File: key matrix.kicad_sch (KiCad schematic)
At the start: 68 parts, among them J3 JST_SUR_SM04B-SURS-TF, J4 JST_SUR_SM04B-SURS-TF, SW1 SW_Push, SW10 SW_Push, SW11 SW_Push, SW12 SW_Push, SW13 SW_Push, SW14 SW_Push, SW15 SW_Push, SW16 SW_Push, SW17 SW_Push, SW18 SW_Push, SW19 SW_Push, SW2 SW_Push, SW20 SW_Push, SW21 SW_Push, SW22 SW_Push, SW23 SW_Push, SW24 SW_Push, SW25 SW_Push, SW26 SW_Push, SW27 SW_Push, SW28 SW_Push, SW29 SW_Push, SW3 SW_Push, SW30 SW_Push, SW31 SW_Push, SW32 SW_Push, SW33 SW_Push, SW34 SW_Push, SW35 SW_Push, SW36 SW_Push, SW37 SW_Push, SW38 SW_Push, SW39 SW_Push, SW4 SW_Push, SW40 SW_Push, SW41 SW_Push, SW42 SW_Push, SW43 RotaryEncoder_Switch_MP, SW44 RotaryEncoder_Switch_MP, SW49 SW_rocker, SW5 SW_Push, SW50 SW_rocker, SW6 SW_Push, SW7 SW_Push, SW8 SW_Push, SW9 SW_Push, U1 BAT54CTB6_R1_00001, U10 BAT54CTB6_R1_00001, U11 BAT54CTB6_R1_00001, U12 BAT54CTB6_R1_00001, U2 BAT54CTB6_R1_00001, U3 BAT54CTB6_R1_00001, U4 BAT54CTB6_R1_00001, U5 BAT54CTB6_R1_00001, U6 BAT54CTB6_R1_00001, U7 BAT54CTB6_R1_00001, U8 BAT54CTB6_R1_00001, U9 BAT54CTB6_R1_00001

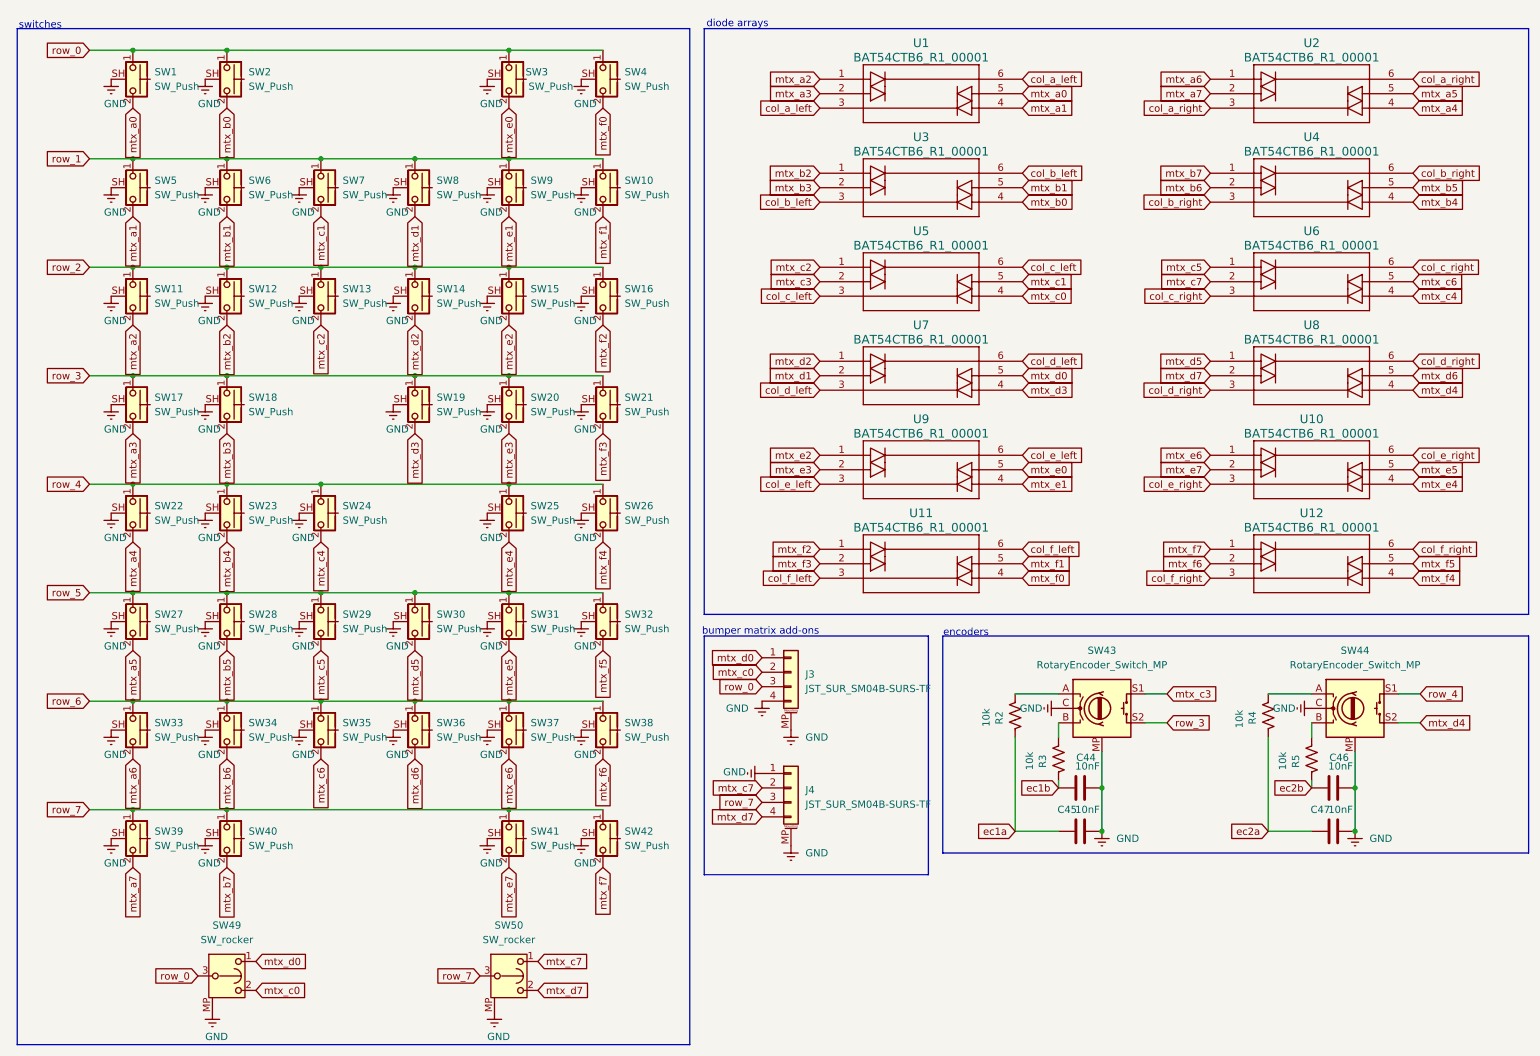
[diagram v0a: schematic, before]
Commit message: v2 final ready to order
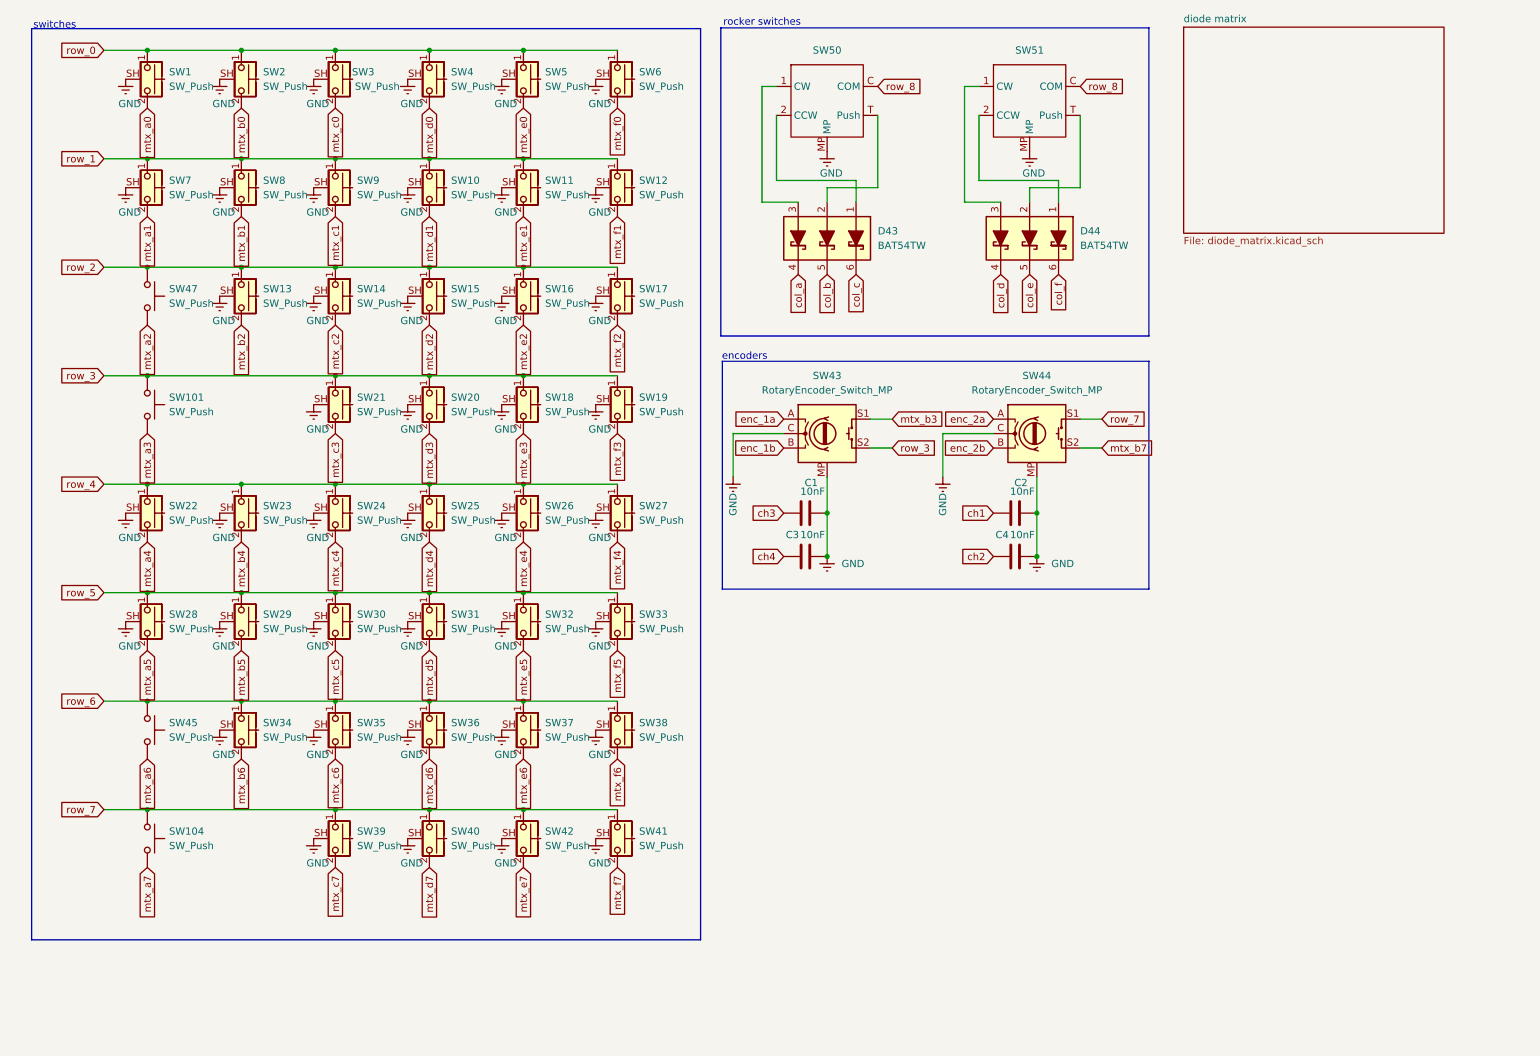
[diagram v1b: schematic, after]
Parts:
- removed C44, C45, C46, C47: 10nF, Capacitor_SMD:C_0603_1608Metric, symbol Device:C
- removed J3, J4: JST_SUR_SM04B-SURS-TF, Connector_JST:JST_SUR_SM04B-SURS-TF_1x04-1MP_P0.80mm_Horizontal, symbol Connector_Generic_MountingPin:Conn_01x04_MountingPin
- removed R2, R3, R4, R5: 10k, Resistor_SMD:R_0603_1608Metric, symbol Device:R_US
- removed SW49, SW50: SW_rocker, coquette_footprints:TMHU27, symbol coquette_symbols:SW_rocker
- removed U1, U10, U11, U12, U2, U3, U4, U5, U6, U7, U8, U9: BAT54CTB6_R1_00001, Package_TO_SOT_SMD:SOT-563, symbol coquette_symbols:BAT54CTB6_R1_00001
- added C1, C2, C3, C4: 10nF, Capacitor_SMD:C_0603_1608Metric, symbol Device:C
- added D43, D44: BAT54TW, PCM_Package_TO_SOT_SMD_AKL:SOT-363_SC-70-6, symbol PCM_Diode_Schottky_AKL:BAT54TW
- added SW101, SW104, SW45, SW47: SW_Push, coquette_footprints:G-Switch GT-TC041B-H036-L1N, symbol Switch:SW_Push
- added SW50, SW51: ~, coquette_footprints:Hanbo WS003, symbol gachlilit:WS-003
- renumbered SW11 to SW10, SW12 to SW11, SW13 to SW12, SW14 to SW13, SW15 to SW14, SW16 to SW15, SW18 to SW16, SW19 to SW18, SW20 to SW19, SW21 to SW20, SW4 to SW21, SW23 to SW22, SW24 to SW23, SW22 to SW24, SW42 to SW27, SW27 to SW28, SW28 to SW29, SW29 to SW30, SW30 to SW31, SW31 to SW32, SW32 to SW33, SW33 to SW34, SW34 to SW35, SW35 to SW36, SW36 to SW37, SW37 to SW38, SW38 to SW39, SW5 to SW4, SW39 to SW40, SW40 to SW41, SW41 to SW42, SW6 to SW5, SW7 to SW6, SW8 to SW7, SW9 to SW8, SW10 to SW9
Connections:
- net GND: now also C1.2, C2.2, C3.2, C4.2, SW50.MP, SW51.MP
- net mtx_a1: now also SW7.2; no longer SW4.2
- net mtx_a2: now also SW47.2; no longer SW10.2
- net mtx_a3: now also SW101.2; no longer SW17.2
- net mtx_a4: now also SW22.2; no longer SW24.2
- net mtx_a6: now also SW45.2; no longer SW34.2
- net mtx_a7: now also SW104.2; no longer SW40.2
- net mtx_b1: now also SW8.2; no longer SW5.2
- net mtx_b2: now also SW13.2; no longer SW11.2
- net mtx_b3: now also SW43.S1; no longer SW16.2
- net mtx_b4: now also SW23.2; no longer SW22.2
- net mtx_b6: now also SW34.2; no longer SW35.2
- net mtx_b7: now also SW44.S2; no longer SW41.2
- net mtx_c0: now also SW3.2
- net mtx_c1: now also SW9.2; no longer SW6.2
- net mtx_c2: now also SW14.2; no longer SW12.2
- net mtx_c3: now also SW21.2; no longer SW43.S1
- net mtx_c4: now also SW24.2; no longer SW23.2
- net mtx_c6: now also SW35.2; no longer SW36.2
- net mtx_c7: now also SW39.2
- net mtx_d0: now also SW4.2
- net mtx_d1: now also SW10.2; no longer SW7.2
- net mtx_d2: now also SW15.2; no longer SW13.2
- net mtx_d3: now also SW20.2; no longer SW18.2
- net mtx_d4: now also SW25.2; no longer SW44.S2
- net mtx_d6: now also SW36.2; no longer SW37.2
- net mtx_d7: now also SW40.2
- net mtx_e0: now also SW5.2; no longer SW3.2
- net mtx_e1: now also SW11.2; no longer SW8.2
- net mtx_e2: now also SW16.2; no longer SW14.2
- net mtx_e3: now also SW18.2; no longer SW19.2
- net mtx_e4: now also SW26.2; no longer SW25.2
- net mtx_e6: now also SW37.2; no longer SW38.2
- net mtx_f0: now also SW6.2; no longer SW21.2
- net mtx_f1: now also SW12.2; no longer SW9.2
- net mtx_f2: now also SW17.2; no longer SW15.2
- net mtx_f3: now also SW19.2; no longer SW20.2
- net mtx_f4: now also SW27.2; no longer SW26.2
- net mtx_f6: now also SW38.2; no longer SW39.2
- net mtx_f7: now also SW41.2; no longer SW27.2
- net row_0: now also SW4.1, SW5.1, SW6.1; no longer SW21.1
- net row_1: now also SW10.1, SW11.1, SW12.1; no longer SW4.1, SW5.1, SW6.1
- net row_2: now also SW16.1, SW17.1, SW47.1; no longer SW10.1, SW11.1, SW12.1
- net row_3: now also SW21.1, SW101.1; no longer SW16.1, SW17.1
- net row_4: now also SW27.1; no longer SW44.S1
- net row_6: now also SW45.1; no longer SW39.1
- net row_7: now also SW39.1, SW44.S1, SW104.1; no longer SW27.1
- net enc_1b: now reaches SW43.B
- net enc_1a: now reaches SW43.A
- net enc_2b: now reaches SW44.B
- net enc_2a: now reaches SW44.A
- new net: D44.3 (A3), SW51.1 (CW)
- new net: D44.1 (A1), SW51.2 (CCW)
- new net: D44.2 (A2), SW51.T (Push)
- new net: D43.3 (A3), SW50.1 (CW)
- new net: D43.1 (A1), SW50.2 (CCW)
- new net: D43.2 (A2), SW50.T (Push)
- new net ch1: C2.1
- new net ch2: C4.1
- new net ch3: C1.1
- new net ch4: C3.1
- new net col_a: D43.4 (K3)
- new net col_b: D43.5 (K2)
- new net col_c: D43.6 (K1)
- new net col_d: D44.4 (K3)
- new net col_e: D44.5 (K2)
- new net col_f: D44.6 (K1)
- new net row_8: SW50.C (COM), SW51.C (COM)
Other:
- added sheet diode matrix (diode_matrix.kicad_sch)
- note added: "rocker switches"
- note removed: "bumper matrix add-ons"
- note removed: "diode arrays"
- moved on the sheet: SW1, SW10, SW11, SW12, SW13, SW14, SW15, SW16, SW17, SW18, SW19, SW2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
